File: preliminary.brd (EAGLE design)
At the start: 79.5 x 77.5 mm, 70 parts, among them IC1 STM32F407VGT6, J3 POWER_JACK, Q1 600mA/40V, U1 STMPS2141STR, Y1 8MHz

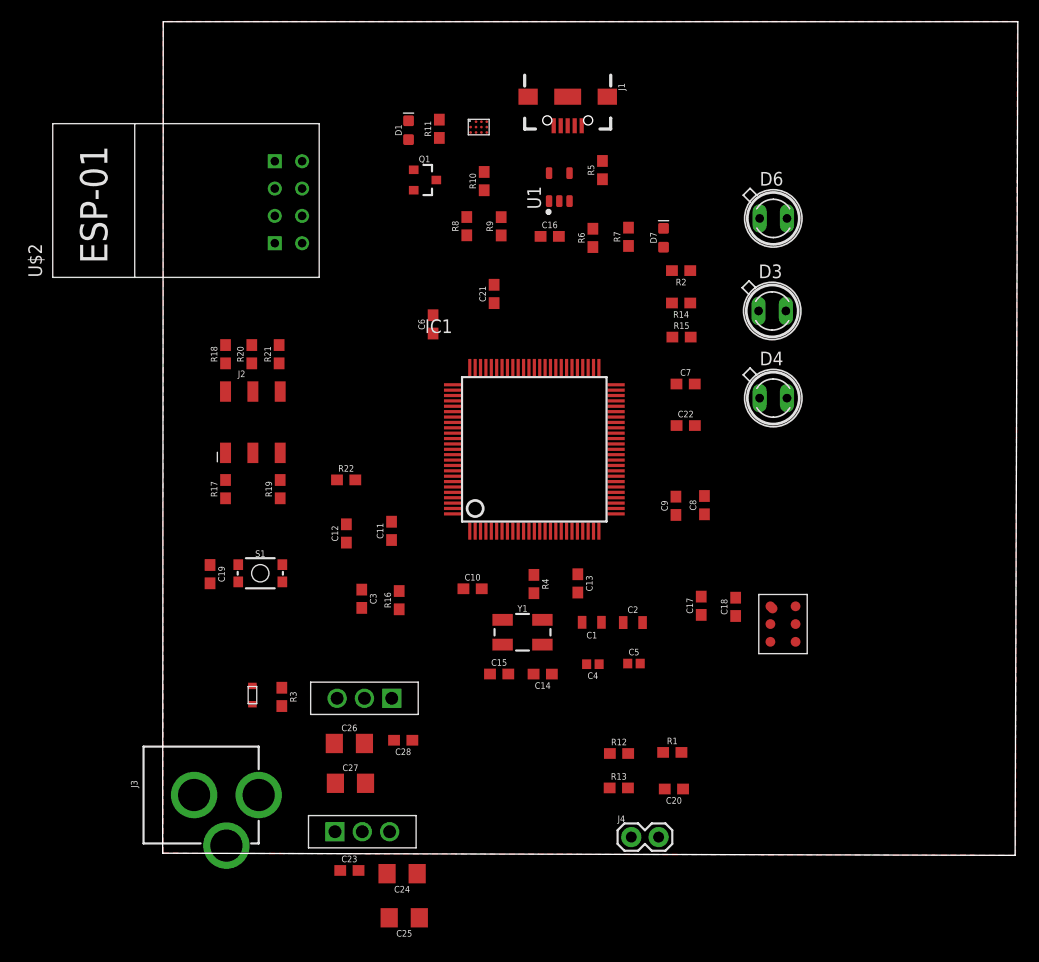
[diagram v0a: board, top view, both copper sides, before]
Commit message: 2nd revision finished
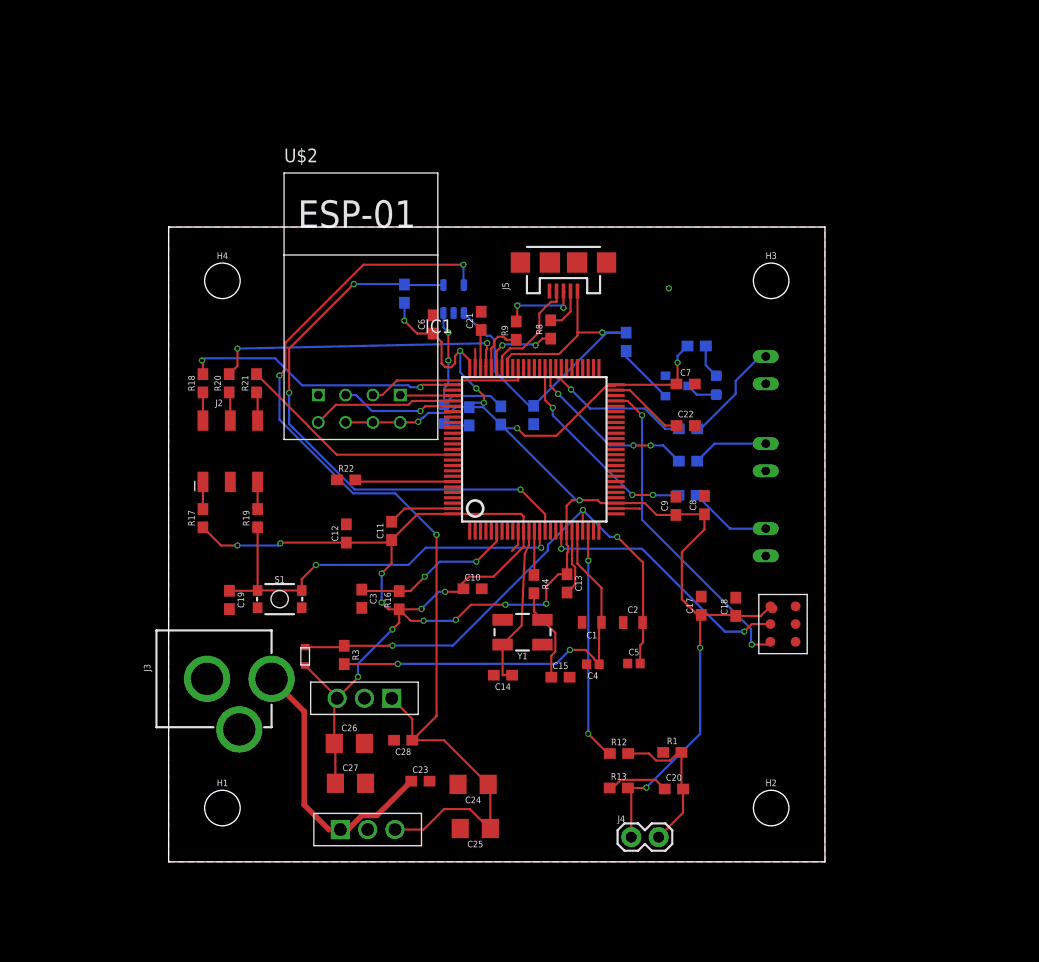
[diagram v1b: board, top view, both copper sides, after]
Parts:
- removed J1: (no value), SparkFun-Connectors:USB-AB-MICRO-SMD
- removed U$3: EMIF02-USB03F2, EMIF02-USB03F2:FLIP-CHIP
- added H1, H2, H3, H4: STAND-OFF, SparkFun-Hardware:STAND-OFF
- added J5: (no value), SparkFun-Connectors:USB-MICROB
- moved D1 37.1 mm to (63.9, 59.3), flipped to the bottom, turned to 270 degrees
- moved R11 31.3 mm to (62.1, 62.9), flipped to the bottom, turned to 0 degrees
- moved Q1 30.2 mm to (60.2, 59.2), flipped to the bottom, turned to 90 degrees
- moved D7 26.2 mm to (38.6, 56.6), flipped to the bottom
- moved R7 22.3 mm to (40.9, 56.4), flipped to the bottom, turned to 270 degrees
- moved R5 21.7 mm to (34.9, 67.8), flipped to the bottom, turned to 270 degrees
- moved R10 19.9 mm to (55.5, 63.3), flipped to the bottom, turned to 270 degrees
- moved R6 18.6 mm to (43.9, 56.5), flipped to the bottom
- moved U$2 18.3 mm to (30.7, 64.0), turned to 0 degrees
- moved C16 16.7 mm to (46.9, 56.5), flipped to the bottom, turned to 90 degrees
- moved R2 14.7 mm to (61.3, 55.2), flipped to the bottom, turned to 0 degrees
- moved R14 14.7 mm to (61.3, 52.2), flipped to the bottom, turned to 0 degrees
- moved R15 14.7 mm to (61.2, 49.1), flipped to the bottom
- moved U1 14.3 mm to (39.5, 67.3), flipped to the bottom
- moved D6 14.1 mm to (68.5, 60.7), flipped to the bottom, turned to 270 degrees
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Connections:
- removed net VDD: C17.1, C18.1, U$6.VDD1, U$6.VDD2
- net +3V3: now also C17.1, C18.1, U$6.VDD1, U$6.VDD2
- net +5V: now also U$5.P$1
- net GND: now also J5.GND; no longer J1.GND1, J1.SHLD1, J1.SHLD2, J1.SHLD3, U$3.11
- net N$6: now also J5.D-; no longer J1.D-1, U$3.10
- net N$7: now also J5.D+; no longer J1.D+1, U$3.7
- net PA10: now also J5.ID; no longer J1.ID1, U$3.3
- net PA11: no longer U$3.12
- net PA12: no longer U$3.9
- net PA9: now also J5.VBUS; no longer J1.VBUS1, U$3.6
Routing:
- net +3V3: track 0.00 -> 230.3 mm, vias 0 -> 22
- net +5V: track 0.00 -> 95.9 mm, vias 0 -> 3
- net PC0: track 0.00 -> 52.9 mm, vias 0 -> 3
- net VDDA: track 0.00 -> 50.9 mm, vias 0 -> 3
- net PA9: track 0.00 -> 40.3 mm, vias 0 -> 1
- net NRST: track 0.00 -> 38.7 mm, vias 0 -> 2
- net VREF+: track 0.00 -> 38.2 mm, vias 0 -> 2
- net PB10: track 0.00 -> 30.3 mm, vias 0 -> 2
- net PA13: track 0.00 -> 28.3 mm, vias 0 -> 2
- net PA14: track 0.00 -> 25.9 mm, vias 0 -> 2
- net N$23: track 0.00 -> 25.7 mm
- net PC3: track 0.00 -> 24.7 mm, vias 0 -> 2
- net PA0: track 0.00 -> 21.6 mm, vias 0 -> 2
- net PB3: track 0.00 -> 21.3 mm
- net N$13: track 0.00 -> 19.5 mm, vias 0 -> 3
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- added copper zone on layer 16, net GND
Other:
- board size 79.5 x 77.5 mm -> 61 x 59 mm
